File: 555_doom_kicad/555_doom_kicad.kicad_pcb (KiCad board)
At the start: 4 copper layers, 92.7 x 63 mm, 89 parts, among them J1 Power, J2 Speaker, Q1 2N3904, Q2 2N3904, SW1 SW_Push, U1 NE555P, U2 74LS161, U3 74154, U4 74HC14, U5 CD4066BE, U6 CD4066BE, U7 NE555P, U8 LM386

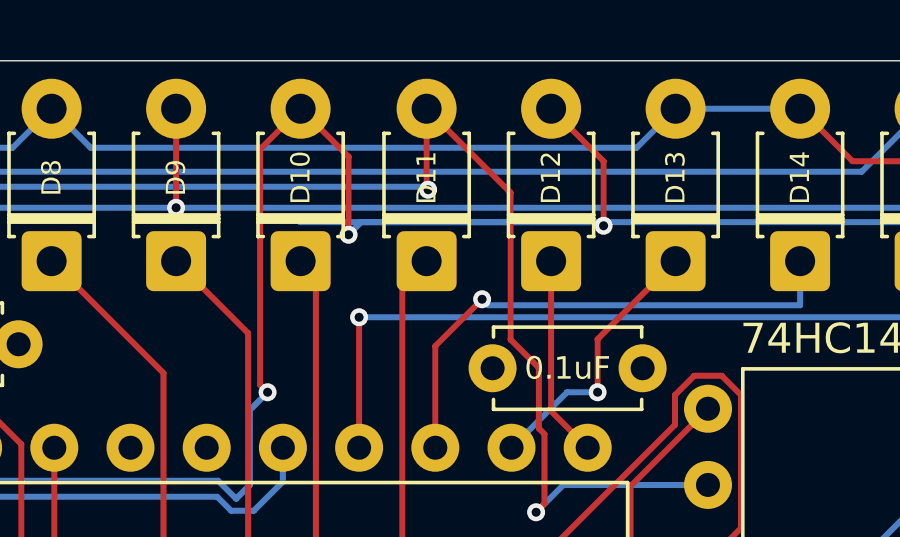
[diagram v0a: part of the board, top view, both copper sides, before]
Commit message: Add KiCad files.
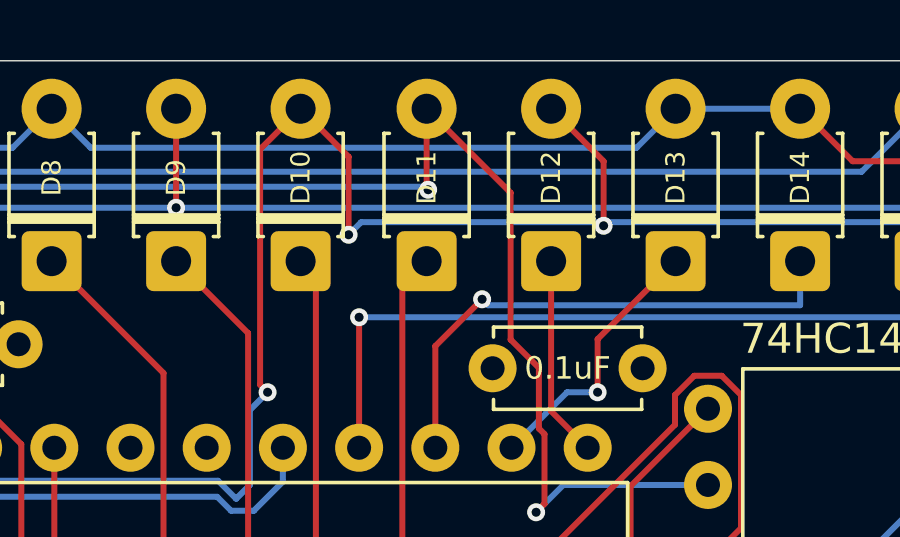
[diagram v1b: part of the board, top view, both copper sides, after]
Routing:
- net /B2: track 94.7 -> 84.7 mm
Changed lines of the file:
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@@
 			(plot_on_all_layers_selection 0x00000000_00000000_00000000_00000000)
 			(disableapertmacros no)
-			(usegerberextensions no)
+			(usegerberextensions yes)
 			(usegerberattributes yes)
 			(usegerberadvancedattributes yes)
@@
 			(outputformat 1)
 			(mirror no)
-			(drillshape 1)
+			(drillshape 0)
 			(scaleselection 1)
-			(outputdirectory "")
+			(outputdirectory "gerber/")
 		)
 	)
@@
 	)
 	(segment
-		(start 206.8 110.08)
-		(end 206.78 110.08)
-		(width 0.2)
-		(layer "B.Cu")
-		(net "/B2")
-	)
-	(segment
 		(start 208.82 110.08)
 		(end 216.78 110.08)
@@
 		(width 0.2)
 		(layer "B.Cu")
-		(net "/B2")
-	)
-	(segment
-		(start 216.78 110.08)
-		(end 206.8 110.08)
-		(width 0.2)
-		(layer "B.Cu")
